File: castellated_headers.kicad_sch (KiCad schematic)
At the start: 4 parts, among them J5 Conn_01x22, J7 Conn_01x22, J8 Conn_01x22, J9 Conn_01x22

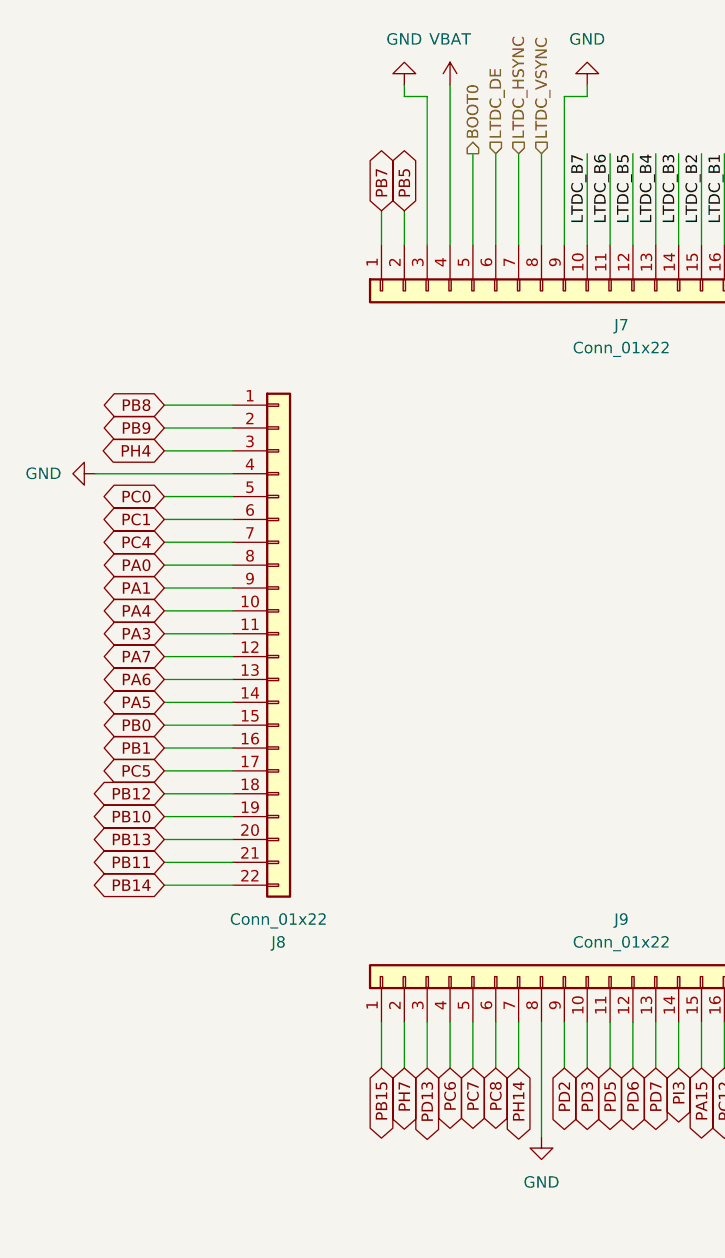
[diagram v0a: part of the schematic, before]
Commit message: generate doc
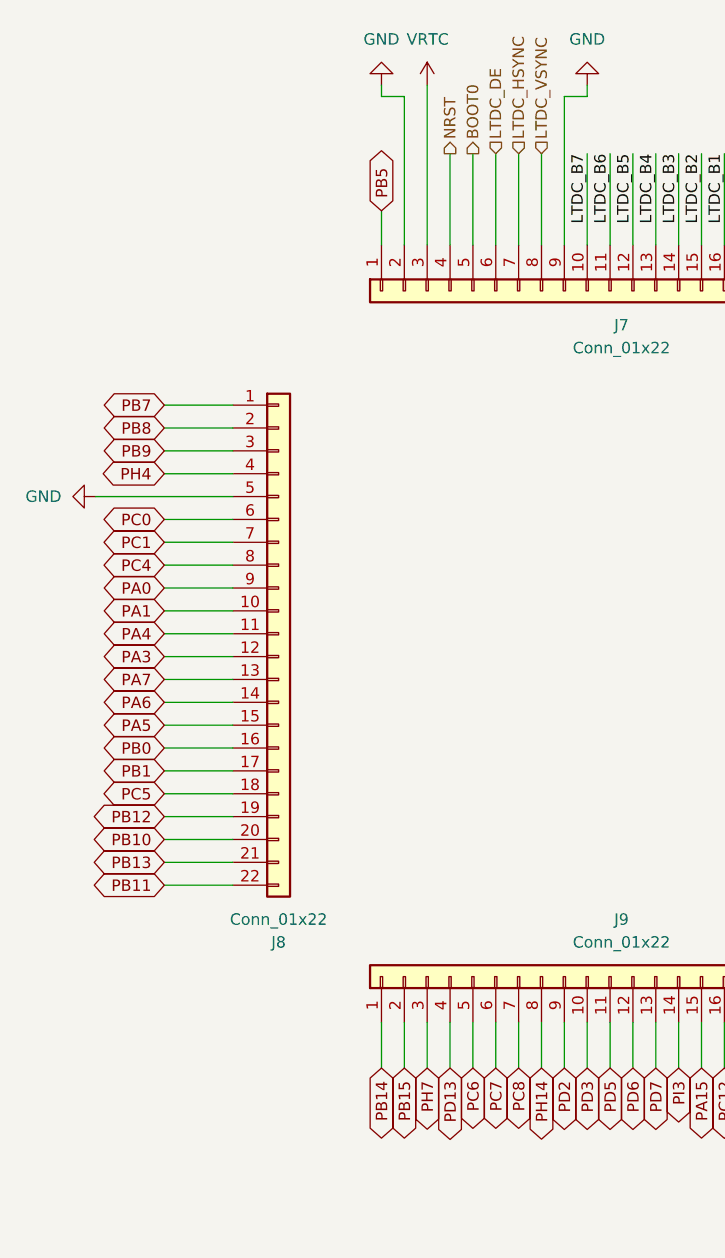
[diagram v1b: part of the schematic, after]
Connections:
- net GND: now also J7.2 (Pin_2), J8.5 (Pin_5); no longer J7.3 (Pin_3), J8.4 (Pin_4), J9.8 (Pin_8)
- net PA0: now also J8.9 (Pin_9); no longer J8.8 (Pin_8)
- net PA1: now also J8.10 (Pin_10); no longer J8.9 (Pin_9)
- net PA3: now also J8.12 (Pin_12); no longer J8.11 (Pin_11)
- net PA4: now also J8.11 (Pin_11); no longer J8.10 (Pin_10)
- net PA5: now also J8.15 (Pin_15); no longer J8.14 (Pin_14)
- net PA6: now also J8.14 (Pin_14); no longer J8.13 (Pin_13)
- net PA7: now also J8.13 (Pin_13); no longer J8.12 (Pin_12)
- net PB0: now also J8.16 (Pin_16); no longer J8.15 (Pin_15)
- net PB1: now also J8.17 (Pin_17); no longer J8.16 (Pin_16)
- net PB10: now also J8.20 (Pin_20); no longer J8.19 (Pin_19)
- net PB11: now also J8.22 (Pin_22); no longer J8.21 (Pin_21)
- net PB12: now also J8.19 (Pin_19); no longer J8.18 (Pin_18)
- net PB13: now also J8.21 (Pin_21); no longer J8.20 (Pin_20)
- net PB14: now also J9.1 (Pin_1); no longer J8.22 (Pin_22)
- net PB15: now also J9.2 (Pin_2); no longer J9.1 (Pin_1)
- net PB5: now also J7.1 (Pin_1); no longer J7.2 (Pin_2)
- net PB7: now also J8.1 (Pin_1); no longer J7.1 (Pin_1)
- net PB8: now also J8.2 (Pin_2); no longer J8.1 (Pin_1)
- net PB9: now also J8.3 (Pin_3); no longer J8.2 (Pin_2)
- net PC0: now also J8.6 (Pin_6); no longer J8.5 (Pin_5)
- net PC1: now also J8.7 (Pin_7); no longer J8.6 (Pin_6)
- net PC4: now also J8.8 (Pin_8); no longer J8.7 (Pin_7)
- net PC5: now also J8.18 (Pin_18); no longer J8.17 (Pin_17)
- net PC6: now also J9.5 (Pin_5); no longer J9.4 (Pin_4)
- net PC7: now also J9.6 (Pin_6); no longer J9.5 (Pin_5)
- net PC8: now also J9.7 (Pin_7); no longer J9.6 (Pin_6)
- net PD13: now also J9.4 (Pin_4); no longer J9.3 (Pin_3)
- net PH14: now also J9.8 (Pin_8); no longer J9.7 (Pin_7)
- net PH4: now also J8.4 (Pin_4); no longer J8.3 (Pin_3)
- net PH7: now also J9.3 (Pin_3); no longer J9.2 (Pin_2)
- net VBAT renamed NRST
- new net VRTC: J7.3 (Pin_3)
